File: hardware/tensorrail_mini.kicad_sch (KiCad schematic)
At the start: 37 parts, among them J1 GCT USB4135-GF-A, J2 Feather Header Left, J3 Feather Header Right, J4 JTAG 2x5, J5 Expansion 2x10, U1 TPS62130ARGTR, U2 TPS62130ARGTR, U3 INA219AIDCNT, U4 W25Q128JVSIQ, U5 APS6404L-3SQR, U6 CH340C

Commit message: Polish hardware signoff artifacts
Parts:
- removed C5, C6, C7, C8: 100nF, Capacitor_SMD:C_0402_1005Metric, symbol Device:C
- removed LED1: Green, LED_SMD:LED_0402_1005Metric, symbol Device:LED
- removed LED2: Blue, LED_SMD:LED_0402_1005Metric, symbol Device:LED
- removed LED3: Red, LED_SMD:LED_0402_1005Metric, symbol Device:LED
- removed R10: 330, Resistor_SMD:R_0402_1005Metric, symbol Device:R
- added D1: Green, LED_SMD:LED_0402_1005Metric, symbol Device:LED
- added D2: Yellow, LED_SMD:LED_0402_1005Metric, symbol Device:LED
- added D3: Red, LED_SMD:LED_0402_1005Metric, symbol Device:LED
- added R10, R11: 330, Resistor_SMD:R_0402_1005Metric, symbol Device:R
- added R10: 0.1, Resistor_SMD:R_2512_6332Metric, symbol Device:R
- C1, C2, C3, C4: value 10uF -> 22uF; footprint Capacitor_SMD:C_0402_1005Metric -> Capacitor_SMD:C_0805_2012Metric
- C11: value 22uF -> 100nF; footprint Capacitor_SMD:C_0805_2012Metric -> Capacitor_SMD:C_0402_1005Metric
- J2: value Feather Header Left -> Feather_Left
- J3: value Feather Header Right -> Feather_Right
- J4: value JTAG 2x5 -> JTAG_2x5; footprint Connector_PinHeader_2.54mm:PinHeader_2x05_P2.54mm_Vertical -> Connector_IDC:IDC-Header_2x05_P2.54mm_Horizontal
- J5: value Expansion 2x10 -> Expansion_2x10
- L1, L2: footprint Inductor_SMD:L_Bourns-SRN4018 -> Inductor_SMD:L_0402_1005Metric
- R2: value 100k -> 56.2k
- R3: value 100k -> 200k
- R4: value 100k -> 33.2k
- R5, R6: value 10k -> 5.1k
- R7, R8: value 10k -> 4.7k
- R9: value 0.1 -> 330; footprint Resistor_SMD:R_0805_2012Metric -> Resistor_SMD:R_0402_1005Metric
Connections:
- net +1V2: now also C4.1, L2.1, R3.1, U2.12 (BOOT), U2.13 (VOS), U3.1 (IN+), U3.2 (IN-), R10.1, R10.2
- net +3V3: now also C11.1, C2.1, C3.1, C9.1, J2.1 (Pin1), J3.1 (Pin1), J4.1 (VCC), J5.1 (P1), L1.1, L1.2, R1.1, R7.1, R8.1, R9.1, U1.10 (SW), U1.11 (SW), U1.12 (BOOT), U1.13 (VOS), U1.9 (SW), U2.1 (VIN), U2.2 (VIN), U2.3 (EN), U3.7 (VS), U4.3 (/WP), U4.7 (/HOLD), U4.8 (VCC), U5.8 (VCC), U6.16 (VCC), R10.1, R11.1
- net GND: now also C1.2, C10.2, C11.2, C2.2, C3.2, C4.2, C9.2, J1.A1/B1 (GND), J1.A12/B12 (GND), J2.16 (Pin16), J2.2 (Pin2), J3.16 (Pin16), J3.2 (Pin2), J4.3 (GND), J4.5 (GND), J4.9 (GND), J5.2 (P2), R2.2, R4.2, R5.2, R6.2, U1.17 (EPAD), U1.7 (GND), U1.8 (GND), U2.17 (EPAD), U2.7 (GND), U2.8 (GND), U3.5 (A0), U3.6 (A1), U3.8 (GND), U4.4 (GND), U5.4 (GND), U6.9 (GND), D1.2 (K), D2.2 (K), D3.2 (K)
- net SCL: now also J2.11 (Pin11), J2.12 (Pin12), R7.2, R8.2, U3.3 (SDA), U3.4 (SCL)
- net SPI_MISO: now also J2.7 (Pin7), U4.2 (DO(MISO)), U5.2 (SO/SIO1)
- net SPI_MOSI: now also J2.6 (Pin6), U4.5 (DI(MOSI)), U5.7 (SI/SIO0)
- net SPI_SCK: now also J2.5 (Pin5), U4.6 (CLK), U5.6 (SCLK)
- net VBUS_RAW: now also C1.1, J1.A4/B4 (VBUS), J1.A9/B9 (VBUS), U1.1 (VIN), U1.2 (VIN), U1.3 (EN)
- net at R4.1: now also R3.2, U2.6 (FB)
- net at R6.1: now also J1.B5 (CC2)
- net UART_RX: now reaches J2.10 (Pin10)
- net UART_RX: now also U6.3 (RXD)
- net CLK_50M: now reaches J2.13 (Pin13)
- net RESET_N: now reaches J2.3 (Pin3)
- net BOOT_N: now reaches J2.4 (Pin4)
- net FLASH_CS_N: now reaches J2.8 (Pin8)
- net FLASH_CS_N: now also U4.1 (/CS)
- net UART_TX: now reaches J2.9 (Pin9)
- net UART_TX: now also U6.2 (TXD)
- net JTAG_nRST: now reaches J4.10 (RESET)
- net JTAG_TMS: now reaches J4.2 (TMS)
- net JTAG_TCK: now reaches J4.4 (TCK)
- net JTAG_TDO: now reaches J4.6 (TDO)
- net JTAG_TDI: now reaches J4.8 (TDI)
- net at U2.10 (SW): now also L2.2, U2.11 (SW), U2.9 (SW)
- net at U1.6 (FB): now also R1.2, R2.1
- net at U6.4 (V3): now also C10.1
- net at R5.1: now also J1.A5 (CC1)
- net at R9.2: now also D1.1 (A)
- net PSRAM_CS_N: now reaches U5.1 (/CE)
- new net: D2.1 (A), R10.2
- new net: D3.1 (A), R11.2
- no-connect marks 21 -> 62
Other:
- note added: "1.2V RAIL (U2)"
- note added: "2x10 expansion header Status LEDs D1-D3 (330R) Unused pins NC"
- note added: "2x5 JTAG/SWD header JTAG_TCK/TMS/TDI/TDO/nRST"
- note added: "3.3V RAIL (U1)"
- note added: "CH340C UART bridge footprint UART_TX/RX exposed to FPGA/header domain UD+/UD- NC in this power-only USB-C revision"
- note added: "EXPANSION + LEDs (J5)"
- note added: "FLASH + PSRAM"
- note added: "FPGA MODULE (J2/J3)"
- note added: "INA219 +1V2 rail monitor 0.1 Ohm shunt → 320mA FS I2C 0x40 — SDA/SCL to FPGA"
- note added: "JTAG DEBUG (J4)"
- note added: "OrangeCrab 85F ECP5 Feather 2x16 0.1-inch pin headers (3.3V I/O)"
- note added: "POWER INPUT"
- note added: "TELEMETRY (U3)"
- note added: "UART BRIDGE (U6)"
- note added: "USB-C 5V sink only - no USB data CC1/CC2 each use 5.1k Rd to GND; D+/D-/SBU are NC"
- note added: "VIN=+3V3 VOUT=+1V2 @ 1A (FPGA core) FB: R3/R4 divider L2=2.2uH Cout=2x22uF"
- note added: "VIN=VBUS_RAW VOUT=+3V3 @ 2A FB: R1/R2 divider L1=2.2uH Cout=2x22uF"
- note added: "W25Q128 128Mb NOR flash — SPI 20MHz APS6404L 32Mb PSRAM — SPI quad-I/O"

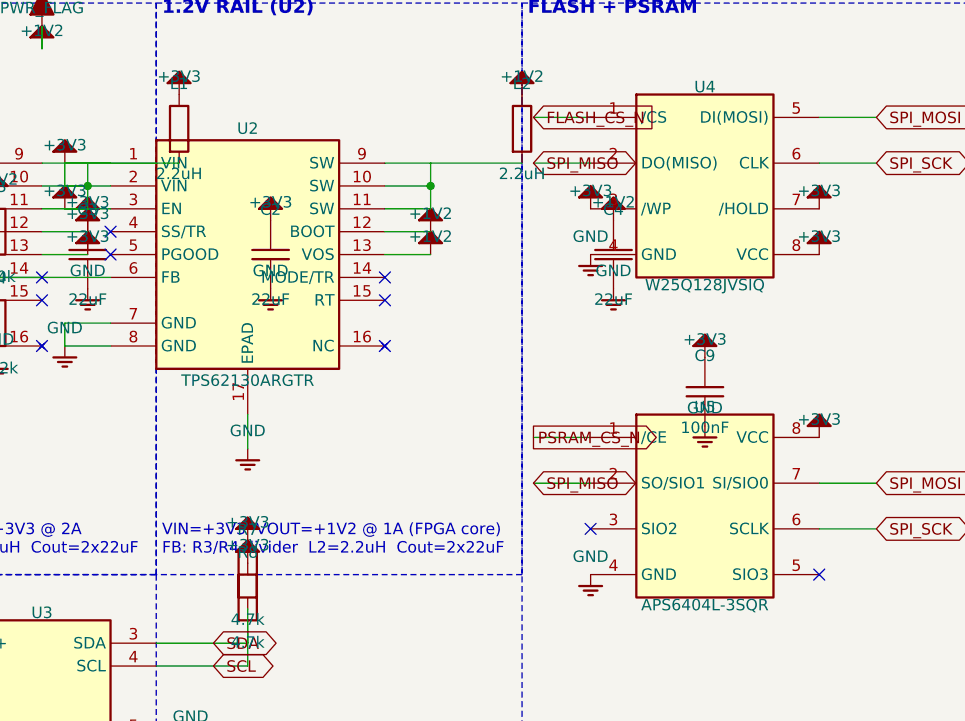
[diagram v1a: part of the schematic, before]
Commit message: Align simulation artifacts with hardware design
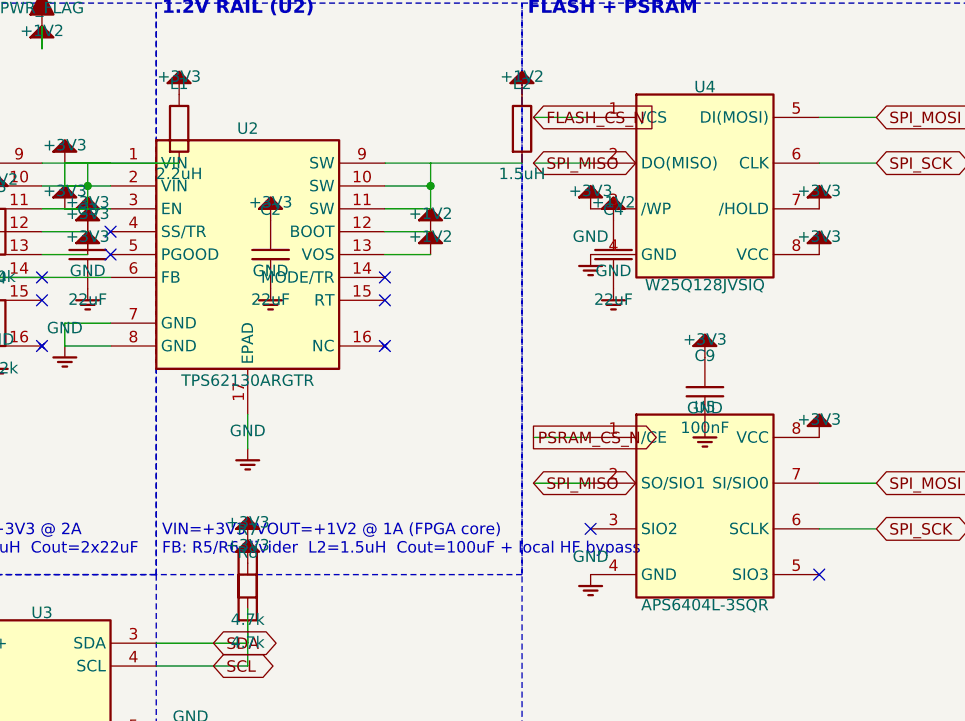
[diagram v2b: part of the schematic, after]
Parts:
- L2: value 2.2uH -> 1.5uH
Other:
- note added: "VIN=+3V3 VOUT=+1V2 @ 1A (FPGA core) FB: R5/R6 divider L2=1.5uH Cout=100uF + local HF bypass"
- note removed: "VIN=+3V3 VOUT=+1V2 @ 1A (FPGA core) FB: R3/R4 divider L2=2.2uH Cout=2x22uF"
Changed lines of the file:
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@@
 		(effects (font (size 1.5 1.5) bold) (justify left))
 	)
-	(text "VIN=+3V3  VOUT=+1V2 @ 1A (FPGA core)\nFB: R3/R4 divider  L2=2.2uH  Cout=2x22uF"
+	(text "VIN=+3V3  VOUT=+1V2 @ 1A (FPGA core)\nFB: R5/R6 divider  L2=1.5uH  Cout=100uF + local HF bypass"
 		(at 89.535 62.23 0)
 		(effects (font (size 1.27 1.27)) (justify left))
@@
 			(effects (font (size 1.27 1.27)))
 		)
-		(property "Value" "2.2uH" (at 129.54 21.51 0)
-			(effects (font (size 1.27 1.27)))
-		)
+		(property "Value" "1.5uH" (at 129.54 21.51 0)
+			(effects (font (size 1.27 1.27)))
+		)
